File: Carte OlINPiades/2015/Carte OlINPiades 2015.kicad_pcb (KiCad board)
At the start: 2 copper layers, 283 parts, among them U1 dsPIC33FJ128MC802, U2 LM7805, U3 LM2937-3.3

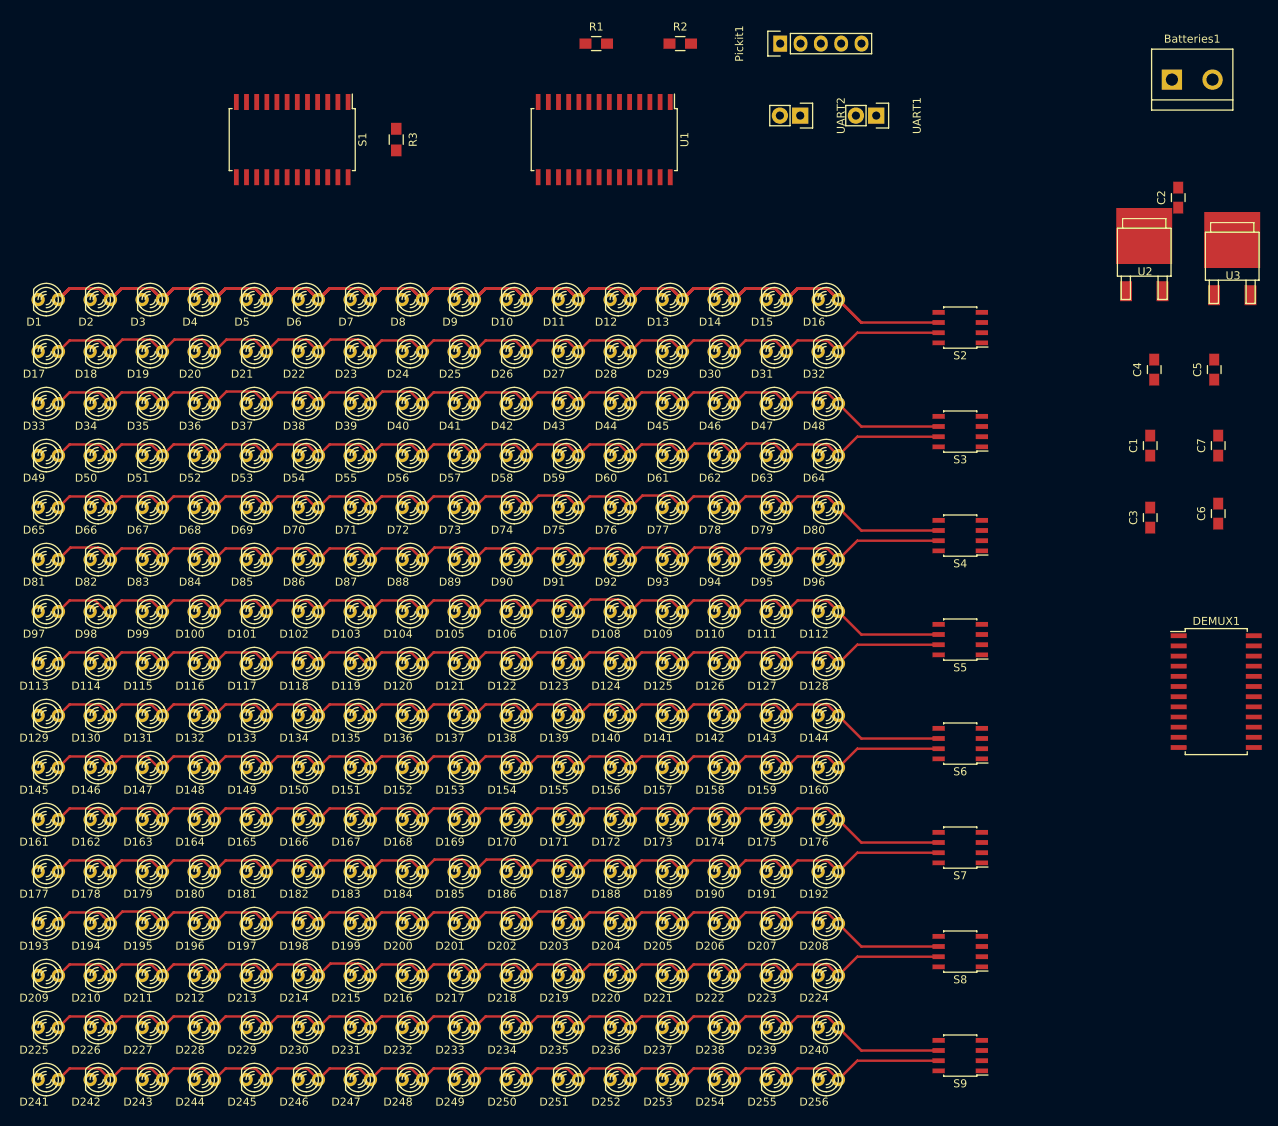
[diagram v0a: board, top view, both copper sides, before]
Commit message: ajoute l'autre face de piste de leds
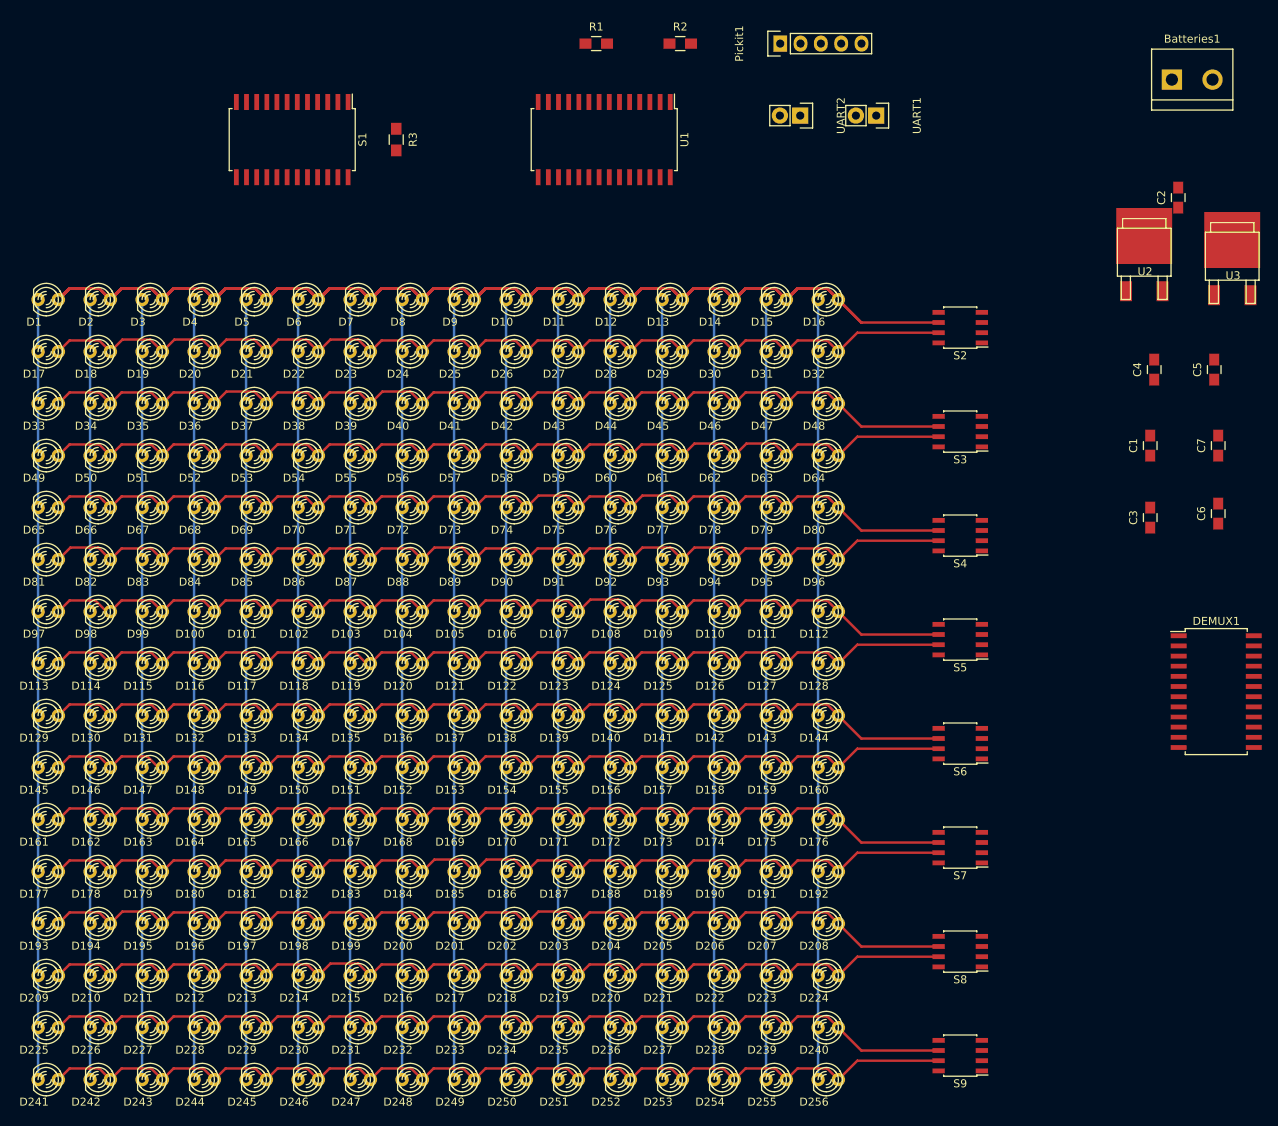
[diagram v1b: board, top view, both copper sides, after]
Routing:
- net Net-(D115-Pad2): track 0.00 -> 97.5 mm
- net Net-(D114-Pad2): track 0.00 -> 97.5 mm
- net Net-(D112-Pad2): track 0.00 -> 97.5 mm
- net Net-(D111-Pad2): track 0.00 -> 97.5 mm
- net Net-(D110-Pad2): track 0.00 -> 97.5 mm
- net Net-(D109-Pad2): track 0.00 -> 97.5 mm
- net Net-(D108-Pad2): track 0.00 -> 97.5 mm
- net Net-(D107-Pad2): track 0.00 -> 97.5 mm
- net Net-(D105-Pad2): track 0.00 -> 97.5 mm
- net Net-(D104-Pad2): track 0.00 -> 97.5 mm
- net Net-(D103-Pad2): track 0.00 -> 97.5 mm
- net Net-(D102-Pad2): track 0.00 -> 97.5 mm
- net Net-(D101-Pad2): track 0.00 -> 97.5 mm
- net Net-(D100-Pad2): track 0.00 -> 97.5 mm
- net Net-(D10-Pad2): track 0.00 -> 97.5 mm
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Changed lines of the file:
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@@
     (thickness 1.6)
     (drawings 0)
-    (tracks 1174)
+    (tracks 1191)
     (zones 0)
     (modules 283)
@@
   (segment (start 149.135 66.865) (end 146.27 64) (width 0.308) (layer F.Cu) (net 6))
   (segment (start 158.8 66.865) (end 149.135 66.865) (width 0.308) (layer F.Cu) (net 6))
+  (segment (start 46.23 64) (end 46.23 161.5) (width 0.308) (layer B.Cu) (net 7))
+  (segment (start 52.73 161.5) (end 52.73 64) (width 0.308) (layer B.Cu) (net 8))
+  (segment (start 59.23 64) (end 59.23 161.5) (width 0.308) (layer B.Cu) (net 9))
+  (segment (start 65.73 161.5) (end 65.73 64) (width 0.308) (layer B.Cu) (net 10))
+  (segment (start 72.23 64) (end 72.23 161.5) (width 0.308) (layer B.Cu) (net 11))
+  (segment (start 78.73 161.5) (end 78.73 64) (width 0.308) (layer B.Cu) (net 12))
+  (segment (start 85.23 64) (end 85.23 161.5) (width 0.308) (layer B.Cu) (net 13))
+  (segment (start 91.73 161.5) (end 91.73 64) (width 0.308) (layer B.Cu) (net 14))
+  (segment (start 98.23 64) (end 98.23 161.5) (width 0.308) (layer B.Cu) (net 15))
+  (segment (start 104.73 161.5) (end 104.73 64) (width 0.308) (layer B.Cu) (net 16))
+  (segment (start 111.23 64) (end 111.23 161.5) (width 0.308) (layer B.Cu) (net 17))
+  (segment (start 117.73 161.5) (end 117.73 64) (width 0.308) (layer B.Cu) (net 18))
+  (segment (start 124.23 64) (end 124.23 161.5) (width 0.308) (layer B.Cu) (net 19))
+  (segment (start 130.73 161.5) (end 130.73 64) (width 0.308) (layer B.Cu) (net 20))
+  (segment (start 137.23 64) (end 137.23 148.020458) (width 0.308) (layer B.Cu) (net 21))
+  (segment (start 137.23 148.020458) (end 137.23 161.5) (width 0.308) (layer B.Cu) (net 21))
+  (segment (start 143.73 161.5) (end 143.73 64) (width 0.308) (layer B.Cu) (net 22))
   (segment (start 55.27 70.5) (end 53.877799 69.107799) (width 0.308) (layer F.Cu) (net 23))
   (segment (start 53.877799 69.107799) (end 50.162201 69.107799) (width 0.308) (layer F.Cu) (net 23))
